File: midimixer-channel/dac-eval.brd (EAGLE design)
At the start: 100 x 80 mm, 20 parts, among them IC1 NE5534AD

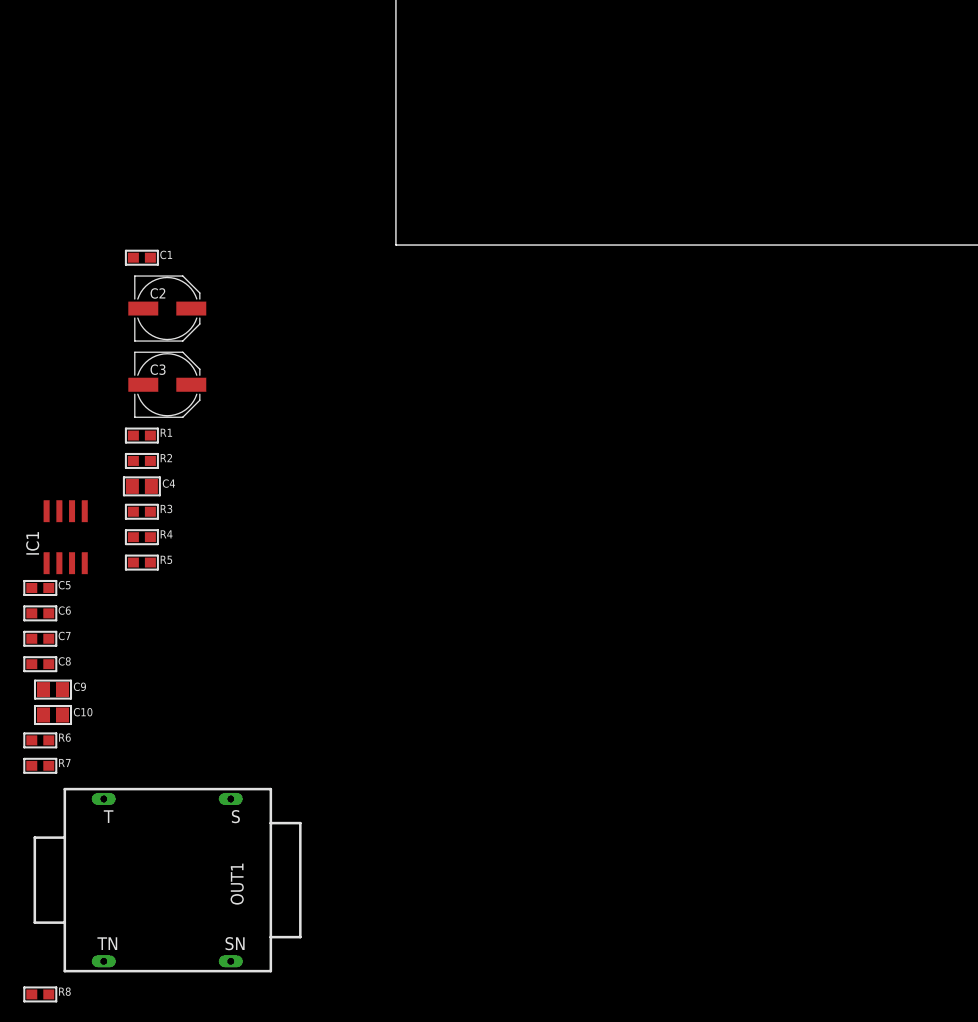
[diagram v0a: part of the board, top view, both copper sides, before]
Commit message: dac wip
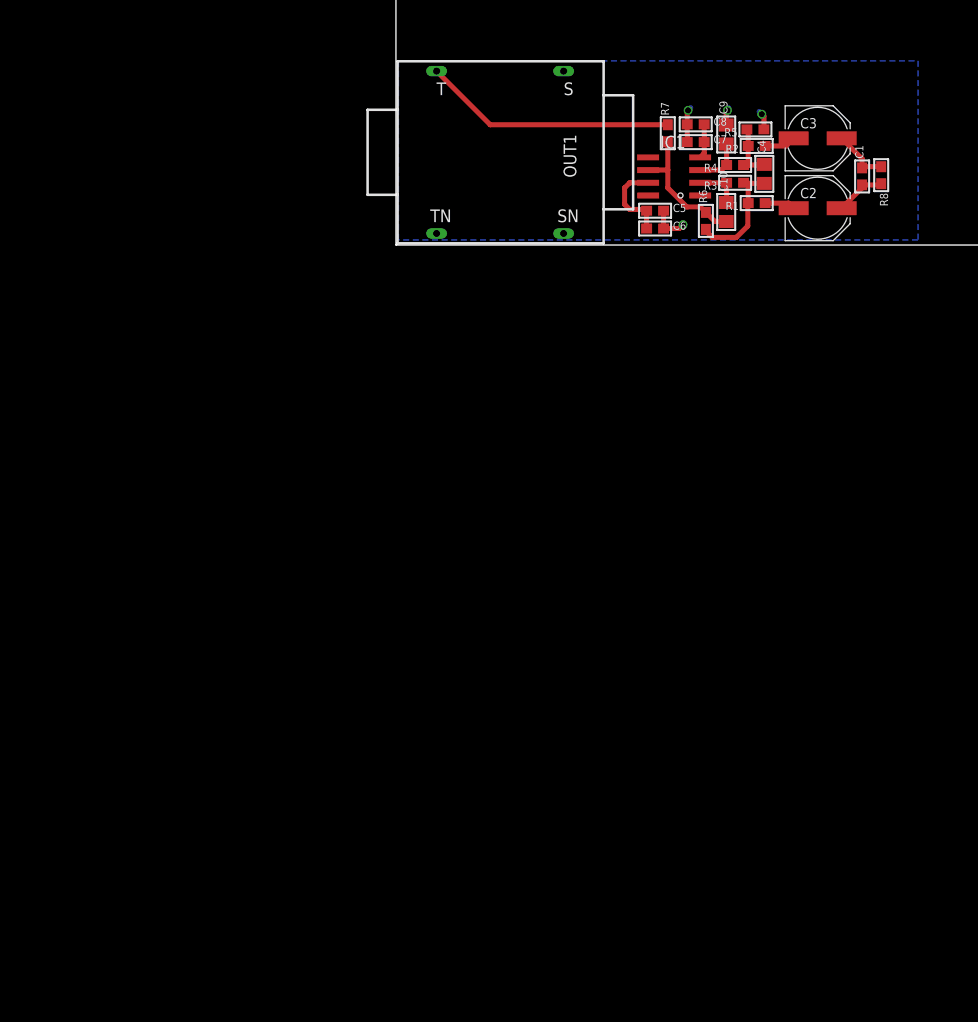
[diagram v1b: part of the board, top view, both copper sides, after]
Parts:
- moved R8 117.4 mm to (48.5, 6.99), turned to 270 degrees
- moved R7 89.1 mm to (27.2, 11.2), turned to 90 degrees
- moved C9 87.2 mm to (33.0, 11.0), turned to 90 degrees
- moved C8 84.9 mm to (30.0, 12.1)
- moved R6 84.4 mm to (31.0, 2.41), turned to 90 degrees
- moved C10 84.0 mm to (33.0, 3.30), turned to 90 degrees
- moved C7 82.2 mm to (30.0, 10.3)
- moved OUT1 80.0 mm to (11.7, 9.27)
- moved R5 75.1 mm to (35.9, 11.6), turned to 180 degrees
- moved C6 72.5 mm to (25.9, 1.65)
- moved C1 72.5 mm to (46.6, 6.86), turned to 90 degrees
- moved C5 72.1 mm to (25.9, 3.43)
- moved IC1 70.7 mm to (27.8, 6.86), turned to 90 degrees
- moved R4 70.0 mm to (33.9, 8.00), turned to 180 degrees
- moved C4 69.6 mm to (36.8, 7.11), turned to 90 degrees
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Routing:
- net N$12: track 0.00 -> 25.3 mm
- net N$10: track 0.00 -> 13.8 mm
- net N$6: track 0.00 -> 11.5 mm
- net AGND: track 0.00 -> 11.4 mm, vias 0 -> 4
- net +12V: track 0.00 -> 8.45 mm
- net OUT1+: track 0.00 -> 5.76 mm
- net N$5: track 0.00 -> 5.74 mm
- net OUT1-: track 0.00 -> 5.13 mm
- net N$8: track 0.00 -> 4.97 mm
- net N$9: track 0.00 -> 4.63 mm
- net -12V: track 0.00 -> 3.47 mm
- net N$4: track 0.00 -> 3.16 mm
- net N$3: track 0.00 -> 3.06 mm
- added copper zone on layer 16, net AGND
